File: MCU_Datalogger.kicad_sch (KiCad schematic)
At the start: 25 parts, among them U1 24LC1025, U2 24LC1025, U3 DS1337S_, U4 ATMEGA328P-AU, Y1 32.768 KHz, Y2 16 MHz

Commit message: Footprints
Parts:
- BT1: footprint (none) -> Connector_PinHeader_2.54mm:PinHeader_1x02_P2.54mm_Vertical
- C1, C2, C3, C4, C5: footprint (none) -> Capacitor_SMD:C_0805_2012Metric_Pad1.18x1.45mm_HandSolder
- D1, D2: footprint (none) -> LED_SMD:LED_0805_2012Metric_Pad1.15x1.40mm_HandSolder
- H1, H2, H3, H4: footprint (none) -> MountingHole:MountingHole_2.1mm
- R1, R2, R3, R4, R5, R6, R7: footprint (none) -> Resistor_SMD:R_0805_2012Metric_Pad1.20x1.40mm_HandSolder
- U1, U2: footprint (none) -> Package_SO:SOIC-8_5.3x5.3mm_P1.27mm
- U3: footprint DS1337S_:SOIC127P600X175-8N -> (none)
- U4: footprint ATMEGA328P-AU:QFP80P900X900X120-32N -> (none)
- Y1, Y2: footprint (none) -> Crystal:Crystal_SMD_5032-2Pin_5.0x3.2mm_HandSoldering
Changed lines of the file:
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@@
 			)
 		)
-		(property "Footprint" ""
+		(property "Footprint" "Crystal:Crystal_SMD_5032-2Pin_5.0x3.2mm_HandSoldering"
 			(at 154.94 67.31 0)
 			(effects
@@
 			)
 		)
-		(property "Footprint" ""
+		(property "Footprint" "Capacitor_SMD:C_0805_2012Metric_Pad1.18x1.45mm_HandSolder"
 			(at 125.4252 48.26 0)
 			(effects
@@
 			)
 		)
-		(property "Footprint" ""
+		(property "Footprint" "Capacitor_SMD:C_0805_2012Metric_Pad1.18x1.45mm_HandSolder"
 			(at 138.7348 59.69 0)
 			(effects
@@
 			)
 		)
-		(property "Footprint" ""
+		(property "Footprint" "MountingHole:MountingHole_2.1mm"
 			(at 90.17 161.29 0)
 			(effects
@@
 			)
 		)
-		(property "Footprint" ""
+		(property "Footprint" "Resistor_SMD:R_0805_2012Metric_Pad1.20x1.40mm_HandSolder"
 			(at 31.242 86.36 90)
 			(effects
@@
 			)
 		)
-		(property "Footprint" ""
+		(property "Footprint" "MountingHole:MountingHole_2.1mm"
 			(at 90.17 167.64 0)
 			(effects
@@
 			)
 		)
-		(property "Footprint" ""
+		(property "Footprint" "Package_SO:SOIC-8_5.3x5.3mm_P1.27mm"
 			(at 85.09 110.49 0)
 			(effects
@@
 			)
 		)
-		(property "Footprint" ""
+		(property "Footprint" "Package_SO:SOIC-8_5.3x5.3mm_P1.27mm"
 			(at 55.88 110.49 0)
 			(effects
@@
 			)
 		)
-		(property "Footprint" ""
+		(property "Footprint" "Resistor_SMD:R_0805_2012Metric_Pad1.20x1.40mm_HandSolder"
 			(at 140.97 55.118 90)
 			(effects
@@
 			)
 		)
-		(property "Footprint" ""
+		(property "Footprint" "Capacitor_SMD:C_0805_2012Metric_Pad1.18x1.45mm_HandSolder"
 			(at 235.9152 48.26 0)
 			(effects
@@
 			)
 		)
-		(property "Footprint" ""
+		(property "Footprint" "LED_SMD:LED_0805_2012Metric_Pad1.15x1.40mm_HandSolder"
 			(at 226.06 63.5 0)
 			(effects
@@
 			)
 		)
-		(property "Footprint" "DS1337S_:SOIC127P600X175-8N"
+		(property "Footprint" ""
 			(at 78.74 54.61 0)
 			(effects
@@
 			)
 		)
-		(property "Footprint" ""
+		(property "Footprint" "Resistor_SMD:R_0805_2012Metric_Pad1.20x1.40mm_HandSolder"
 			(at 33.02 99.568 90)
 			(effects
@@
 			)
 		)
-		(property "Footprint" ""
+		(property "Footprint" "MountingHole:MountingHole_2.1mm"
 			(at 90.17 154.94 0)
 			(effects
@@
 			)
 		)
-		(property "Footprint" ""
+		(property "Footprint" "LED_SMD:LED_0805_2012Metric_Pad1.15x1.40mm_HandSolder"
 			(at 161.29 54.61 0)
 			(effects
@@
 			)
 		)
-		(property "Footprint" ""
+		(property "Footprint" "MountingHole:MountingHole_2.1mm"
 			(at 90.17 173.99 0)
 			(effects
@@
 			)
 		)
-		(property "Footprint" ""
+		(property "Footprint" "Resistor_SMD:R_0805_2012Metric_Pad1.20x1.40mm_HandSolder"
 			(at 225.552 78.74 90)
 			(effects
@@
 			)
 		)
-		(property "Footprint" ""
+		(property "Footprint" "Capacitor_SMD:C_0805_2012Metric_Pad1.18x1.45mm_HandSolder"
 			(at 158.4452 41.91 0)
 			(effects
@@
 			)
 		)
-		(property "Footprint" ""
+		(property "Footprint" "Resistor_SMD:R_0805_2012Metric_Pad1.20x1.40mm_HandSolder"
 			(at 151.13 94.488 90)
 			(effects
@@
 			)
 		)
-		(property "Footprint" "ATMEGA328P-AU:QFP80P900X900X120-32N"
+		(property "Footprint" ""
 			(at 200.66 69.85 0)
 			(effects
@@
 			)
 		)
-		(property "Footprint" ""
+		(property "Footprint" "Connector_PinHeader_2.54mm:PinHeader_1x02_P2.54mm_Vertical"
 			(at 259.08 42.926 90)
 			(effects
@@
 			)
 		)
-		(property "Footprint" ""
+		(property "Footprint" "Capacitor_SMD:C_0805_2012Metric_Pad1.18x1.45mm_HandSolder"
 			(at 140.6652 80.01 0)
 			(effects
@@
 			)
 		)
-		(property "Footprint" ""
+		(property "Footprint" "Resistor_SMD:R_0805_2012Metric_Pad1.20x1.40mm_HandSolder"
 			(at 104.902 44.45 90)
 			(effects
@@
 			)
 		)
-		(property "Footprint" ""
+		(property "Footprint" "Crystal:Crystal_SMD_5032-2Pin_5.0x3.2mm_HandSoldering"
 			(at 31.75 48.26 0)
 			(effects
@@
 			)
 		)
-		(property "Footprint" ""
+		(property "Footprint" "Resistor_SMD:R_0805_2012Metric_Pad1.20x1.40mm_HandSolder"
 			(at 113.792 44.45 90)
 			(effects

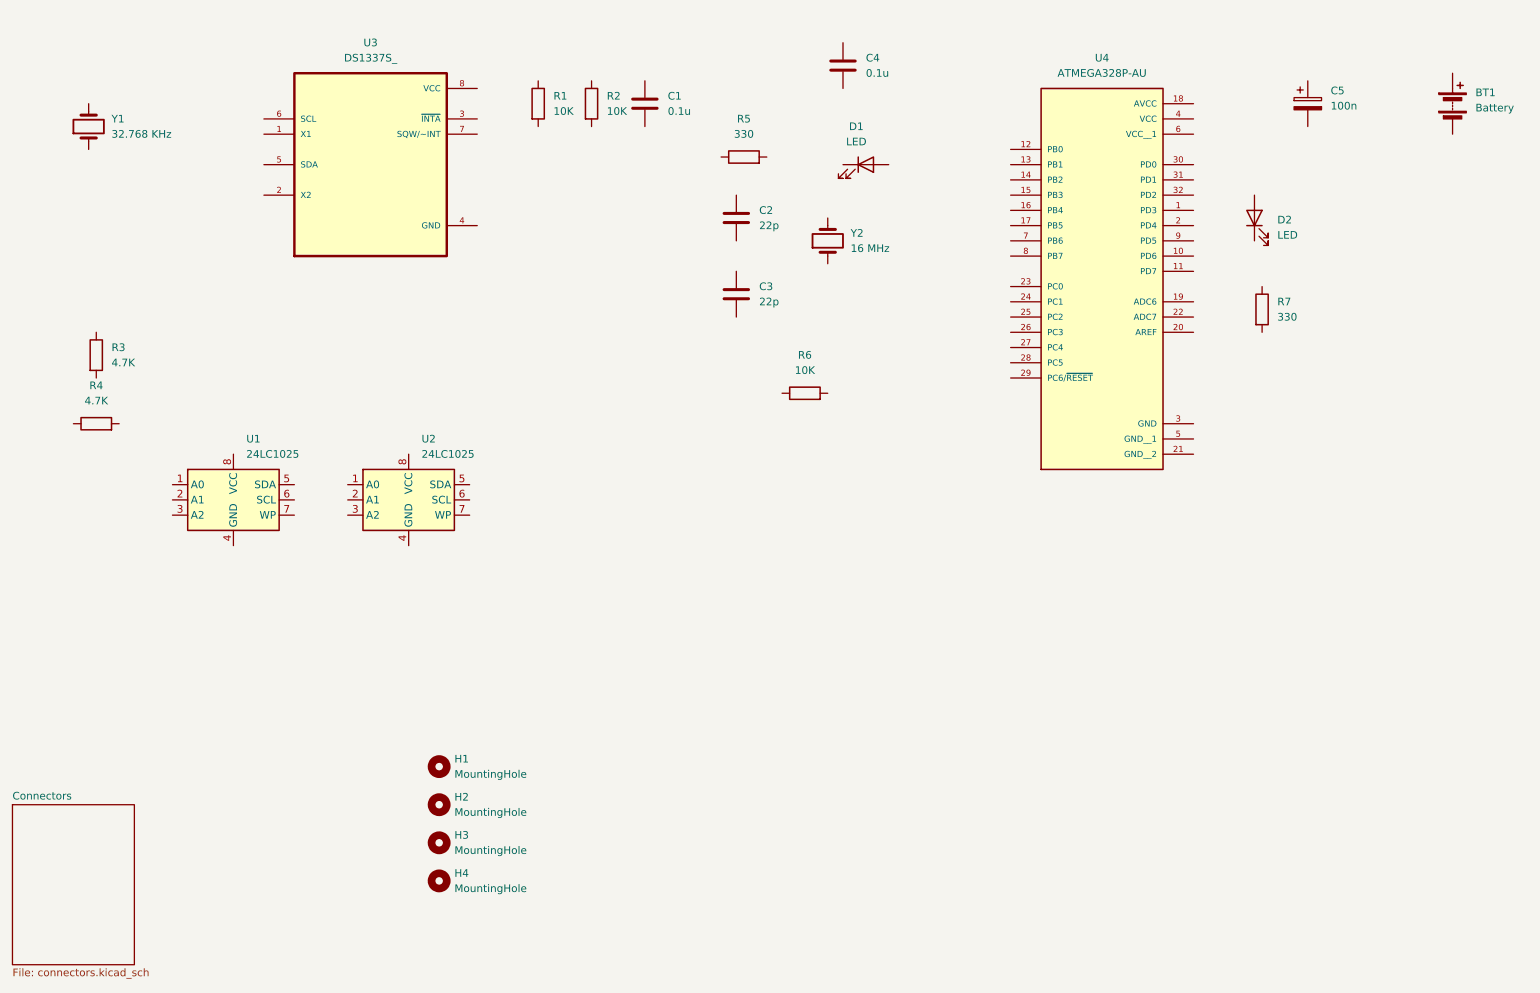
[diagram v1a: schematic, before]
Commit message: Wiring Main
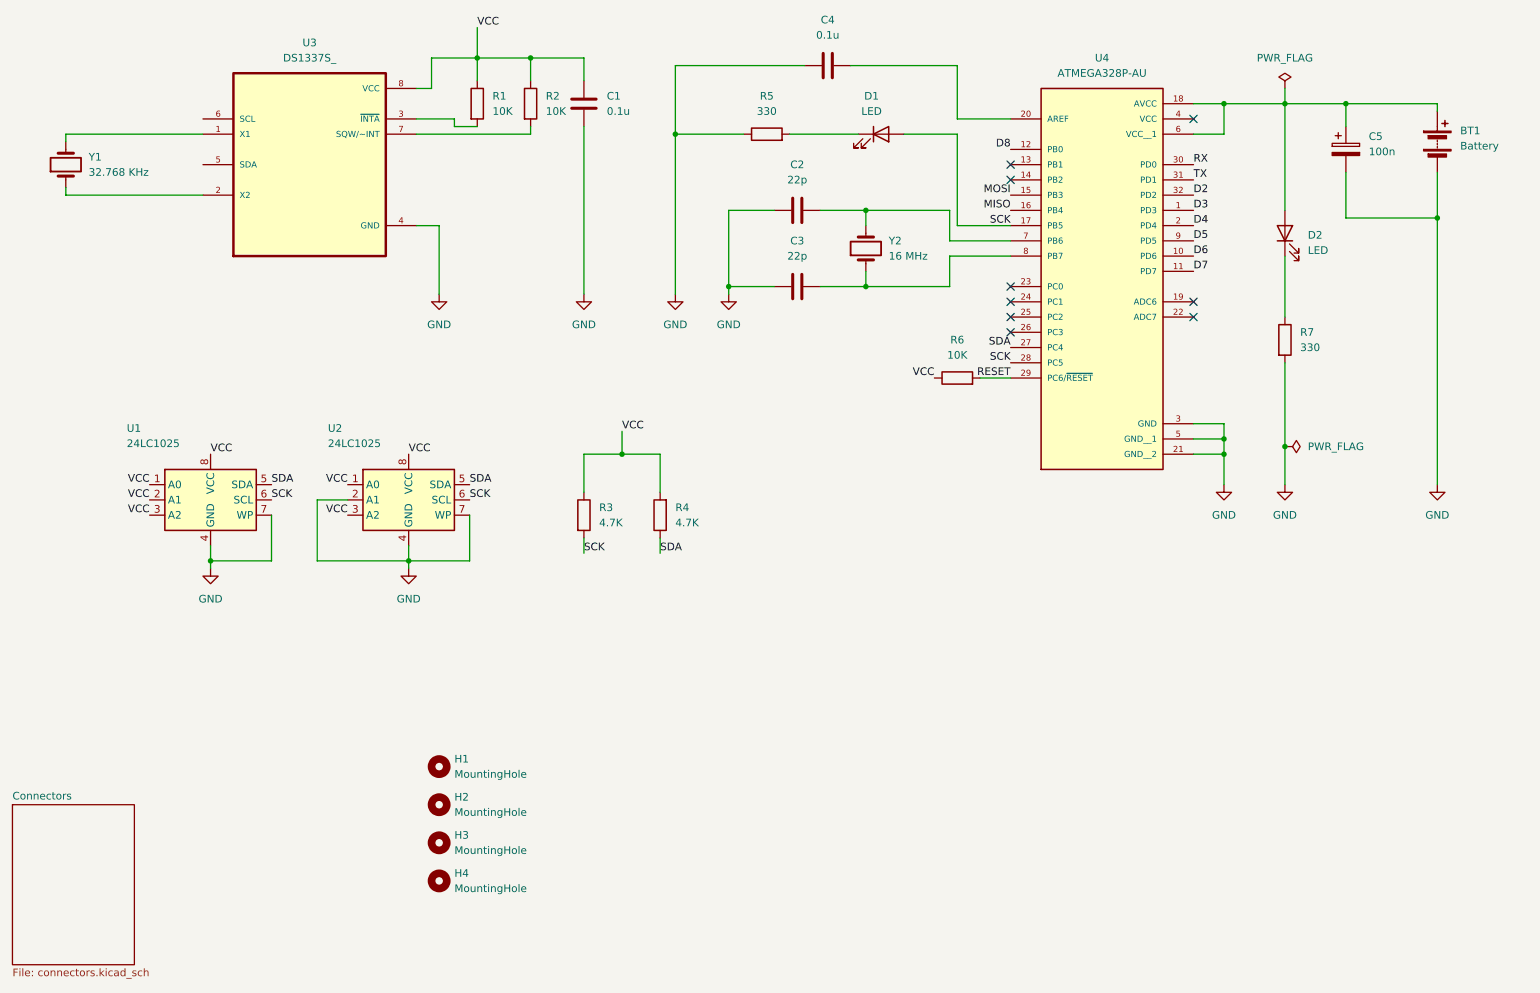
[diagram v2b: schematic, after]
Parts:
- U3: footprint (none) -> DS1337S_:SOIC127P600X175-8N
- U4: footprint (none) -> ATMEGA328P-AU:QFP80P900X900X120-32N
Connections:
- net at Y2.1: now also C3.2, U4.8 (PB7)
- net at Y2.2: now also C2.1, U4.7 (PB6)
- net VCC: now reaches C1.1
- net VCC: now also R1.1, R2.1, R3.1, R4.2, R6.1, U1.1 (A0), U1.2 (A1), U1.3 (A2), U1.8 (VCC), U2.1 (A0), U2.3 (A2), U2.8 (VCC), U3.8 (VCC)
- net GND: now reaches C1.2
- net GND: now also BT1.2 (-), C2.2, C3.1, C4.1, C5.2, R5.1, R7.2, U1.4 (GND), U1.7 (WP), U2.2 (A1), U2.4 (GND), U2.7 (WP), U3.4 (GND), U4.21 (GND__2), U4.3 (GND), U4.5 (GND__1)
- net SCK: now reaches R3.2
- net SCK: now also D1.2 (A), U1.6 (SCL), U2.6 (SCL), U4.17 (PB5), U4.28 (PC5)
- net SDA: now reaches U2.5 (SDA)
- net SDA: now also R4.1, U1.5 (SDA), U4.27 (PC4)
- net at R5.2: now also D1.1 (K)
- net at C5.1: now also BT1.1 (+), D2.2 (A), U4.18 (AVCC), U4.6 (VCC__1)
- net at D2.1 (K): now also R7.1
- net at U3.1 (X1): now also Y1.2
- net at U3.2 (X2): now also Y1.1
- net at U3.3 (~{INTA}): now also R1.2
- net at U3.7 (SQW/~INT): now also R2.2
- net at C4.2: now also U4.20 (AREF)
- net RESET: now reaches R6.2
- net RESET: now also U4.29 (PC6/~{RESET})
- net D3: now reaches U4.1 (PD3)
- net D6: now reaches U4.10 (PD6)
- net D7: now reaches U4.11 (PD7)
- net D8: now reaches U4.12 (PB0)
- net MOSI: now reaches U4.15 (PB3)
- net MISO: now reaches U4.16 (PB4)
- net D4: now reaches U4.2 (PD4)
- net RX: now reaches U4.30 (PD0)
- net TX: now reaches U4.31 (PD1)
- net D2: now reaches U4.32 (PD2)
- net D5: now reaches U4.9 (PD5)
- no-connect marks 0 -> 9
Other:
- moved on the sheet: BT1, C1, C2, C3, C4, C5, D1, D2, R1, R2, R3, R4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
